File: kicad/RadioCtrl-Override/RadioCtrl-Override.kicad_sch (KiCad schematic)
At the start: 17 parts, among them J1 FW/BK/CON, J2 LF/RI/CON, J5 HM10, J6 WRITER, Q1 2SC1815, Q2 2SC1815, Q3 2SC1815, Q4 2SC1815, U1 PIC16F1827-E/P

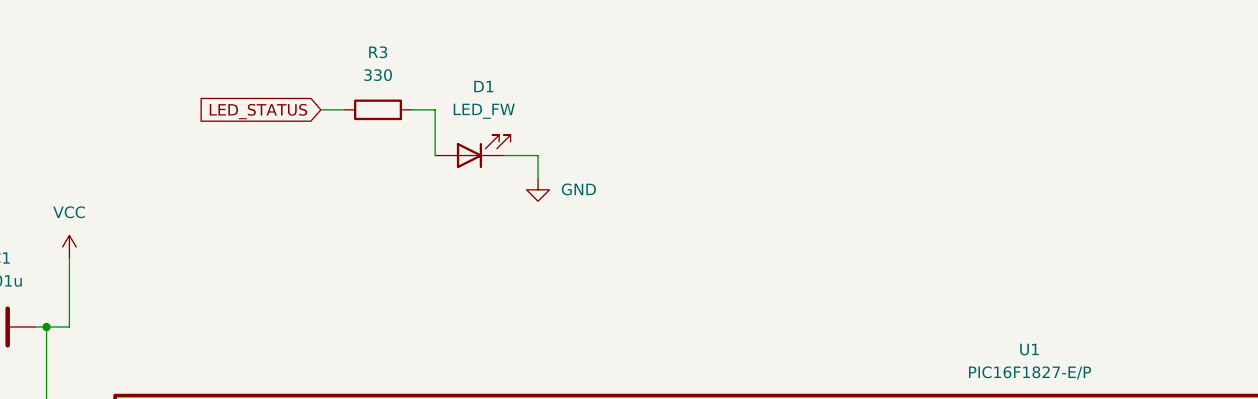
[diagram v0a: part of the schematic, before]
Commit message: pcbレイヤーを作成
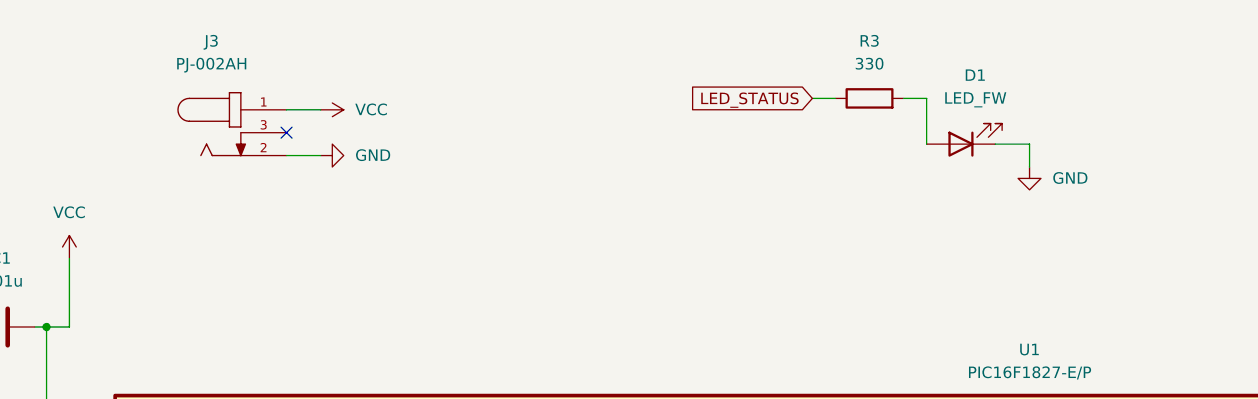
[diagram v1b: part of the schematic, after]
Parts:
- added J3: PJ-002AH, PJ-002AH:CUI_PJ-002AH, symbol PJ-002AH:PJ-002AH
- C1: footprint Capacitor_THT:C_Axial_L3.8mm_D2.6mm_P10.00mm_Horizontal -> Capacitor_THT:C_Disc_D3.0mm_W1.6mm_P2.50mm
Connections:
- net GND: now also J3.2
- net VCC: now also J3.1
- no-connect marks 10 -> 11
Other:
- moved on the sheet: D1, R3
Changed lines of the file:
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@@
   )
   (no_connect (at 40.64 86.36))
+  (no_connect (at 64.77 26.67))
   (no_connect (at 40.64 78.74))
   (no_connect (at 254 71.12))
@@
     (stroke (width 0) (type default) (color 0 0 0 0))
   )
-  (wire (pts (xy 81.28 24.13) (xy 81.28 29.21))
+  (wire (pts (xy 135.89 22.86) (xy 135.89 27.94))
     (stroke (width 0) (type default) (color 0 0 0 0))
   )
@@
     (stroke (width 0) (type default) (color 0 0 0 0))
   )
-  (wire (pts (xy 68.58 24.13) (xy 71.12 24.13))
+  (wire (pts (xy 123.19 22.86) (xy 125.73 22.86))
     (stroke (width 0) (type default) (color 0 0 0 0))
   )
@@
     (stroke (width 0) (type default) (color 0 0 0 0))
   )
-  (wire (pts (xy 88.9 29.21) (xy 92.71 29.21))
+  (wire (pts (xy 64.77 24.13) (xy 68.58 24.13))
+    (stroke (width 0) (type default) (color 0 0 0 0))
+  )
+  (wire (pts (xy 143.51 27.94) (xy 147.32 27.94))
     (stroke (width 0) (type default) (color 0 0 0 0))
   )
@@
     (stroke (width 0) (type default) (color 0 0 0 0))
   )
-  (wire (pts (xy 92.71 29.21) (xy 92.71 31.75))
+  (wire (pts (xy 147.32 27.94) (xy 147.32 30.48))
     (stroke (width 0) (type default) (color 0 0 0 0))
   )
@@
     (stroke (width 0) (type default) (color 0 0 0 0))
   )
+  (wire (pts (xy 64.77 29.21) (xy 68.58 29.21))
+    (stroke (width 0) (type default) (color 0 0 0 0))
+  )
   (wire (pts (xy 255.27 22.86) (xy 256.54 22.86))
     (stroke (width 0) (type default) (color 0 0 0 0))
@@
     (stroke (width 0) (type default) (color 0 0 0 0))
   )
-  (wire (pts (xy 78.74 24.13) (xy 81.28 24.13))
+  (wire (pts (xy 133.35 22.86) (xy 135.89 22.86))
     (stroke (width 0) (type default) (color 0 0 0 0))
   )
@@
     )
   )
-  (global_label "LED_STATUS" (shape input) (at 68.58 24.13 180) (fields_autoplaced)
-    (effects (font (size 1.27 1.27)) (justify right))
-    (property "シート間のリファレンス" "${INTERSHEET_REFS}" (id 0) (at 54.9788 24.0506 0)
+  (global_label "LED_STATUS" (shape input) (at 123.19 22.86 180) (fields_autoplaced)
+    (effects (font (size 1.27 1.27)) (justify right))
+    (property "シート間のリファレンス" "${INTERSHEET_REFS}" (id 0) (at 109.5888 22.7806 0)
       (effects (font (size 1.27 1.27)) (justify right) hide)
     )
@@
       (effects (font (size 1.27 1.27)) (justify right) hide)
     )
+  )
+  (symbol (lib_id "power:GND") (at 68.58 29.21 90) (unit 1)
+    (in_bom yes) (on_board yes) (fields_autoplaced)
+    (property "Reference" "#PWR0106" (id 0) (at 74.93 29.21 0)
+      (effects (font (size 1.27 1.27)) hide)
+    )
+    (property "Value" "GND" (id 1) (at 72.39 29.2099 90)
+      (effects (font (size 1.27 1.27)) (justify right))
+    )
+    (property "Footprint" "" (id 2) (at 68.58 29.21 0)
+      (effects (font (size 1.27 1.27)) hide)
+    )
+    (property "Datasheet" "" (id 3) (at 68.58 29.21 0)
+      (effects (font (size 1.27 1.27)) hide)
+    )
+    (pin "1")
   )
   (symbol (lib_id "Transistor_BJT:2SC1815") (at 208.28 130.81 0) (unit 1)
@@
     (pin "1")
   )
-  (symbol (lib_id "Device:R") (at 74.93 24.13 90) (unit 1)
-    (in_bom yes) (on_board yes) (fields_autoplaced)
-    (property "Reference" "R3" (id 0) (at 74.93 17.78 90))
-    (property "Value" "330" (id 1) (at 74.93 20.32 90))
-    (property "Footprint" "Resistor_THT:R_Axial_DIN0204_L3.6mm_D1.6mm_P2.54mm_Vertical" (id 2) (at 74.93 25.908 90)
-      (effects (font (size 1.27 1.27)) hide)
-    )
-    (property "Datasheet" "~" (id 3) (at 74.93 24.13 0)
+  (symbol (lib_id "Device:R") (at 129.54 22.86 90) (unit 1)
+    (in_bom yes) (on_board yes) (fields_autoplaced)
+    (property "Reference" "R3" (id 0) (at 129.54 16.51 90))
+    (property "Value" "330" (id 1) (at 129.54 19.05 90))
+    (property "Footprint" "Resistor_THT:R_Axial_DIN0204_L3.6mm_D1.6mm_P2.54mm_Vertical" (id 2) (at 129.54 24.638 90)
+      (effects (font (size 1.27 1.27)) hide)
+    )
+    (property "Datasheet" "~" (id 3) (at 129.54 22.86 0)
       (effects (font (size 1.27 1.27)) hide)
     )
@@
     (pin "1")
   )
-  (symbol (lib_id "power:GND") (at 92.71 31.75 0) (unit 1)
-    (in_bom yes) (on_board yes) (fields_autoplaced)
-    (property "Reference" "#PWR06" (id 0) (at 92.71 38.1 0)
-      (effects (font (size 1.27 1.27)) hide)
-    )
-    (property "Value" "GND" (id 1) (at 95.25 33.0199 0)
-      (effects (font (size 1.27 1.27)) (justify left))
-    )
-    (property "Footprint" "" (id 2) (at 92.71 31.75 0)
-      (effects (font (size 1.27 1.27)) hide)
-    )
-    (property "Datasheet" "" (id 3) (at 92.71 31.75 0)
+  (symbol (lib_id "power:GND") (at 147.32 30.48 0) (unit 1)
+    (in_bom yes) (on_board yes) (fields_autoplaced)
+    (property "Reference" "#PWR06" (id 0) (at 147.32 36.83 0)
+      (effects (font (size 1.27 1.27)) hide)
+    )
+    (property "Value" "GND" (id 1) (at 149.86 31.7499 0)
+      (effects (font (size 1.27 1.27)) (justify left))
+    )
+    (property "Footprint" "" (id 2) (at 147.32 30.48 0)
+      (effects (font (size 1.27 1.27)) hide)
+    )
+    (property "Datasheet" "" (id 3) (at 147.32 30.48 0)
       (effects (font (size 1.27 1.27)) hide)
     )
@@
     (pin "2")
     (pin "3")
+  )
+  (symbol (lib_id "power:VCC") (at 68.58 24.13 270) (unit 1)
+    (in_bom yes) (on_board yes) (fields_autoplaced)
+    (property "Reference" "#PWR0105" (id 0) (at 64.77 24.13 0)
+      (effects (font (size 1.27 1.27)) hide)
+    )
+    (property "Value" "VCC" (id 1) (at 72.39 24.1299 90)
+      (effects (font (size 1.27 1.27)) (justify left))
+    )
+    (property "Footprint" "" (id 2) (at 68.58 24.13 0)
+      (effects (font (size 1.27 1.27)) hide)
+    )
+    (property "Datasheet" "" (id 3) (at 68.58 24.13 0)
+      (effects (font (size 1.27 1.27)) hide)
+    )
+    (pin "1")
   )
   (symbol (lib_id "Device:R") (at 198.12 130.81 90) (unit 1)
@@
     (property "Reference" "C1" (id 0) (at 33.02 40.64 90))
     (property "Value" "0.01u" (id 1) (at 33.02 43.18 90))
-    (property "Footprint" "Capacitor_THT:C_Axial_L3.8mm_D2.6mm_P10.00mm_Horizontal" (id 2) (at 36.83 47.2948 0)
+    (property "Footprint" "Capacitor_THT:C_Disc_D3.0mm_W1.6mm_P2.50mm" (id 2) (at 36.83 47.2948 0)
       (effects (font (size 1.27 1.27)) hide)
     )
@@
     (pin "3")
   )
-  (symbol (lib_id "Device:LED") (at 85.09 29.21 180) (unit 1)
-    (in_bom yes) (on_board yes) (fields_autoplaced)
-    (property "Reference" "D1" (id 0) (at 86.6775 21.59 0))
-    (property "Value" "LED_FW" (id 1) (at 86.6775 24.13 0))
-    (property "Footprint" "LED_THT:LED_D3.0mm" (id 2) (at 85.09 29.21 0)
-      (effects (font (size 1.27 1.27)) hide)
-    )
-    (property "Datasheet" "~" (id 3) (at 85.09 29.21 0)
+  (symbol (lib_id "PJ-002AH:PJ-002AH") (at 59.69 26.67 0) (unit 1)
+    (in_bom yes) (on_board yes) (fields_autoplaced)
+    (property "Reference" "J3" (id 0) (at 56.4515 16.51 0))
+    (property "Value" "PJ-002AH" (id 1) (at 56.4515 19.05 0))
+    (property "Footprint" "PJ-002AH:CUI_PJ-002AH" (id 2) (at 59.69 26.67 0)
+      (effects (font (size 1.27 1.27)) (justify bottom) hide)
+    )
+    (property "Datasheet" "" (id 3) (at 59.69 26.67 0)
+      (effects (font (size 1.27 1.27)) hide)
+    )
+    (property "MANUFACTURER" "CUI INC" (id 4) (at 59.69 26.67 0)
+      (effects (font (size 1.27 1.27)) (justify bottom) hide)
+    )
+    (property "STANDARD" "Manufacturer recommendations" (id 5) (at 59.69 26.67 0)
+      (effects (font (size 1.27 1.27)) (justify bottom) hide)
+    )
+    (pin "1")
+    (pin "2")
+    (pin "3")
+  )
+  (symbol (lib_id "Device:LED") (at 139.7 27.94 180) (unit 1)
+    (in_bom yes) (on_board yes) (fields_autoplaced)
+    (property "Reference" "D1" (id 0) (at 141.2875 20.32 0))
+    (property "Value" "LED_FW" (id 1) (at 141.2875 22.86 0))
+    (property "Footprint" "LED_THT:LED_D3.0mm" (id 2) (at 139.7 27.94 0)
+      (effects (font (size 1.27 1.27)) hide)
+    )
+    (property "Datasheet" "~" (id 3) (at 139.7 27.94 0)
       (effects (font (size 1.27 1.27)) hide)
     )
@@
       (reference "#PWR0104") (unit 1) (value "VCC") (footprint "")
     )
+    (path "/b1c3c639-5b8c-4507-b90f-9db0b8c30d9e"
+      (reference "#PWR0105") (unit 1) (value "VCC") (footprint "")
+    )
+    (path "/02c38b03-f119-4b7e-b0ab-f248d95480a0"
+      (reference "#PWR0106") (unit 1) (value "GND") (footprint "")
+    )
     (path "/da3dd5fa-1535-47e6-971b-b4bd7d9cdbdb"
-      (reference "C1") (unit 1) (value "0.01u") (footprint "Capacitor_THT:C_Axial_L3.8mm_D2.6mm_P10.00mm_Horizontal")
+      (reference "C1") (unit 1) (value "0.01u") (footprint "Capacitor_THT:C_Disc_D3.0mm_W1.6mm_P2.50mm")
     )
     (path "/fb7d77e1-5ea3-4ac8-a774-250a84ee9488"
@@
       (reference "J2") (unit 1) (value "LF/RI/CON") (footprint "TerminalBlock_4Ucon:TerminalBlock_4Ucon_1x03_P3.50mm_Horizontal")
     )
+    (path "/e5fbfa3f-ae4a-42b2-a487-5dfbc6ae6990"
+      (reference "J3") (unit 1) (value "PJ-002AH") (footprint "PJ-002AH:CUI_PJ-002AH")
+    )
     (path "/bcd7400f-b002-4e43-92aa-3f85b80fb80a"
